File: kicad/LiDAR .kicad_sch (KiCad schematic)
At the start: 6 parts, among them J17 LiDAR, Q20 AO3400

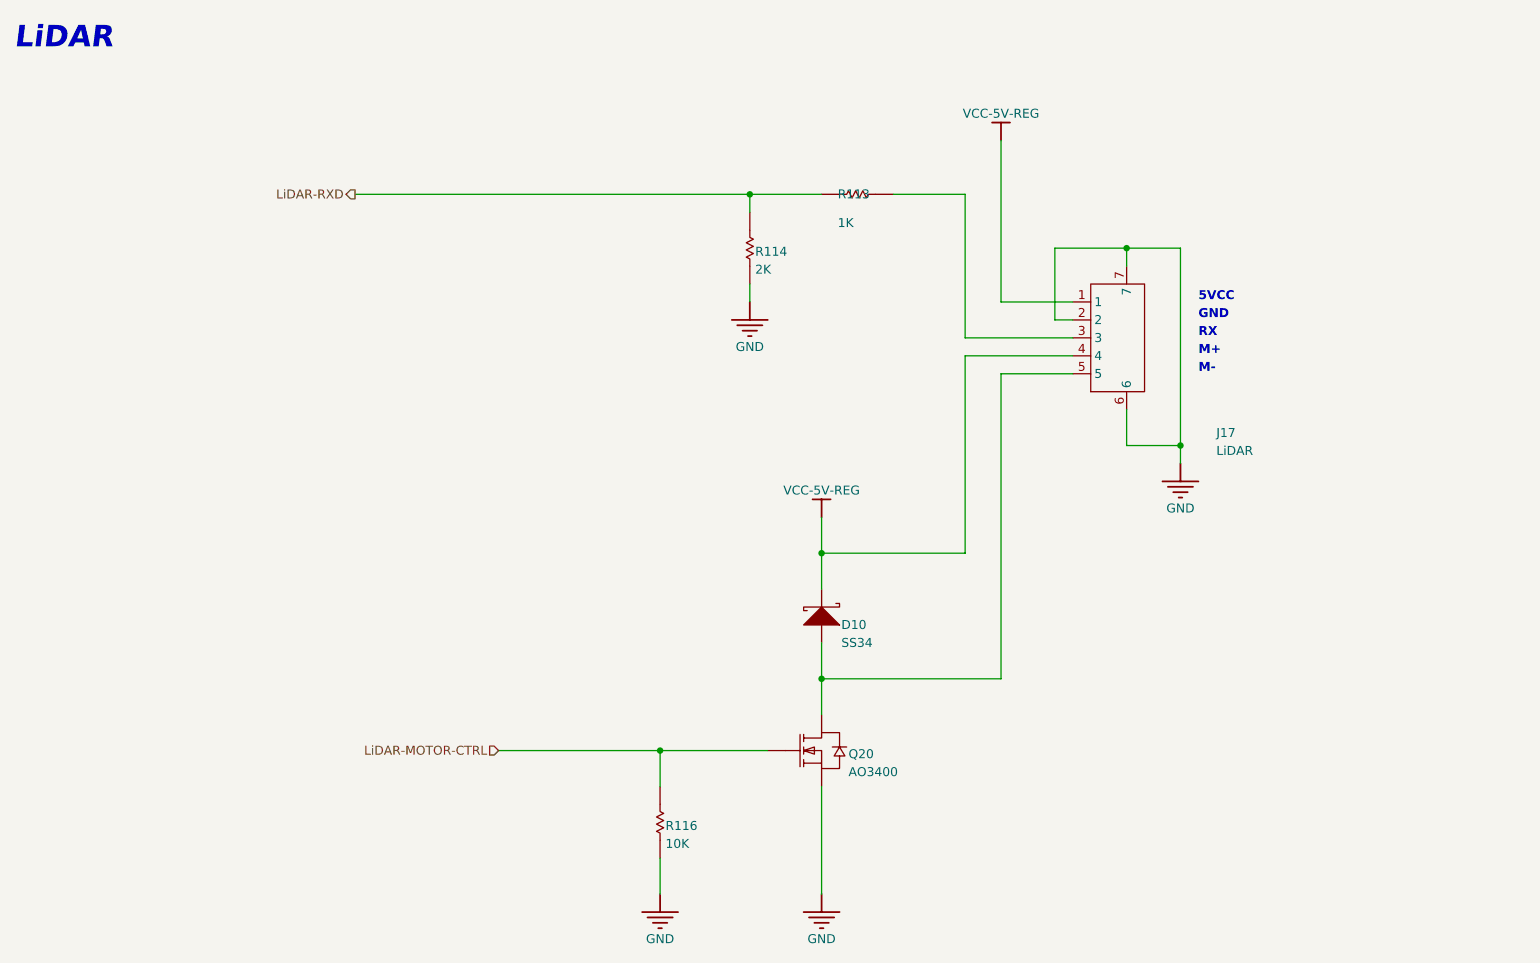
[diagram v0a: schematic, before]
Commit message: STM32G473VCT6
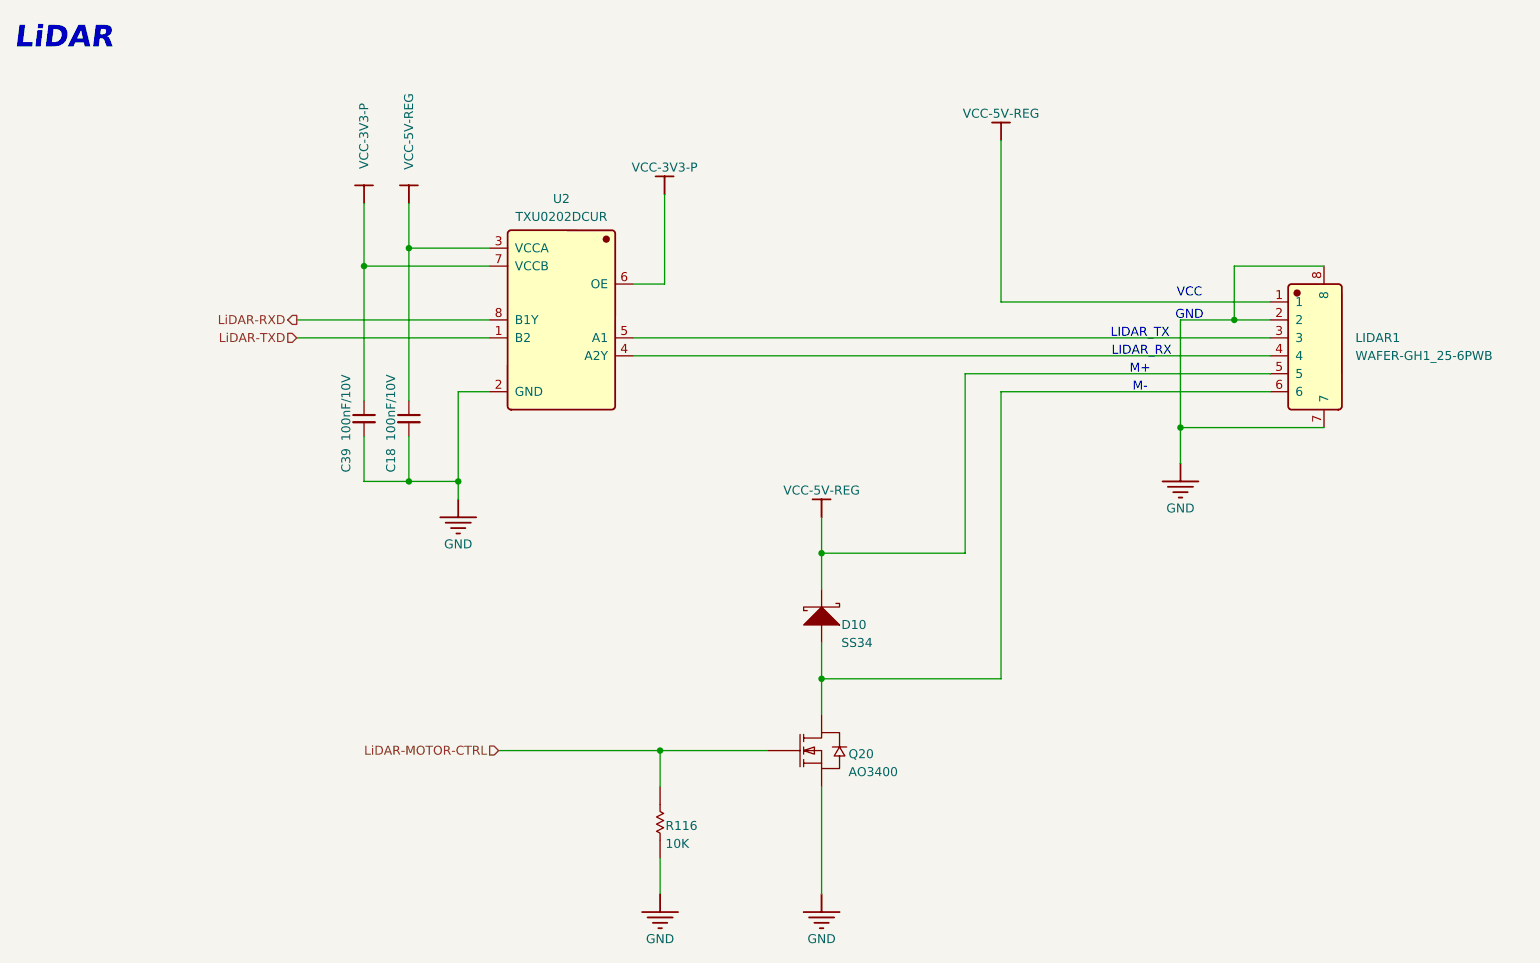
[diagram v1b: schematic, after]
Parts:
- removed J17: LiDAR, oomwoo_altium:CONN-SMD_5P-P1.25_XUNPU_WAFER-GH1.25-5PWB, symbol DesignLibrary:LiDAR_0_HDRx5_DesignLibrary.SchLib
- removed R113: 1K, Resistor_SMD:R_0603_1608Metric, symbol DesignLibrary:LiDAR_0_Resistor-1_DesignLibrary.SchLib
- removed R114: 2K, Resistor_SMD:R_0603_1608Metric, symbol DesignLibrary:LiDAR_1_Resistor-1_DesignLibrary.SchLib
- added C18, C39: 100nF/10V, Capacitor_SMD:C_0603_1608Metric, symbol Device:C_Small
- added LIDAR1: WAFER-GH1_25-6PWB, JLCImport:WAFER-GH1_25-6PWB, symbol JLCImport:WAFER-GH1_25-6PWB
- added U2: TXU0202DCUR, JLCImport:TXU0202DCUR, symbol JLCImport:TXU0202DCUR
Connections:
- net GND: now also C18.2, C39.2, LIDAR1.2, LIDAR1.7, LIDAR1.8, U2.2 (GND)
- net LiDAR-RXD: now also U2.8 (B1Y)
- net VCC-5V-REG: now also C18.1, LIDAR1.1, LIDAR1.5, U2.3 (VCCA)
- net at D10.1 (A), Q20.3 (D): now also LIDAR1.6
- new net: LIDAR1.3, U2.5 (A1)
- new net: LIDAR1.4, U2.4 (A2Y)
- new net LiDAR-TXD: U2.1 (B2)
- new net VCC-3V3-P: C39.1, U2.6 (OE), U2.7 (VCCB)
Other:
- note added: "LIDAR_RX"
- note added: "LIDAR_TX"
- note added: "VCC"
- note removed: "5VCC"
- note removed: "RX"
